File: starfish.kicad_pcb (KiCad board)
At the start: 2 copper layers, 40.5 x 25 mm, 35 parts, among them J1 microUSB, P1 CONN_02X05, P2 CONN_6X2, P3 CONN_2, U1 AP2120N, U2 SAMD21E15A-MU, U3 TPS73101, U4 FXMAR2104, U5 FXMAR2104, X1 CRYSTAL

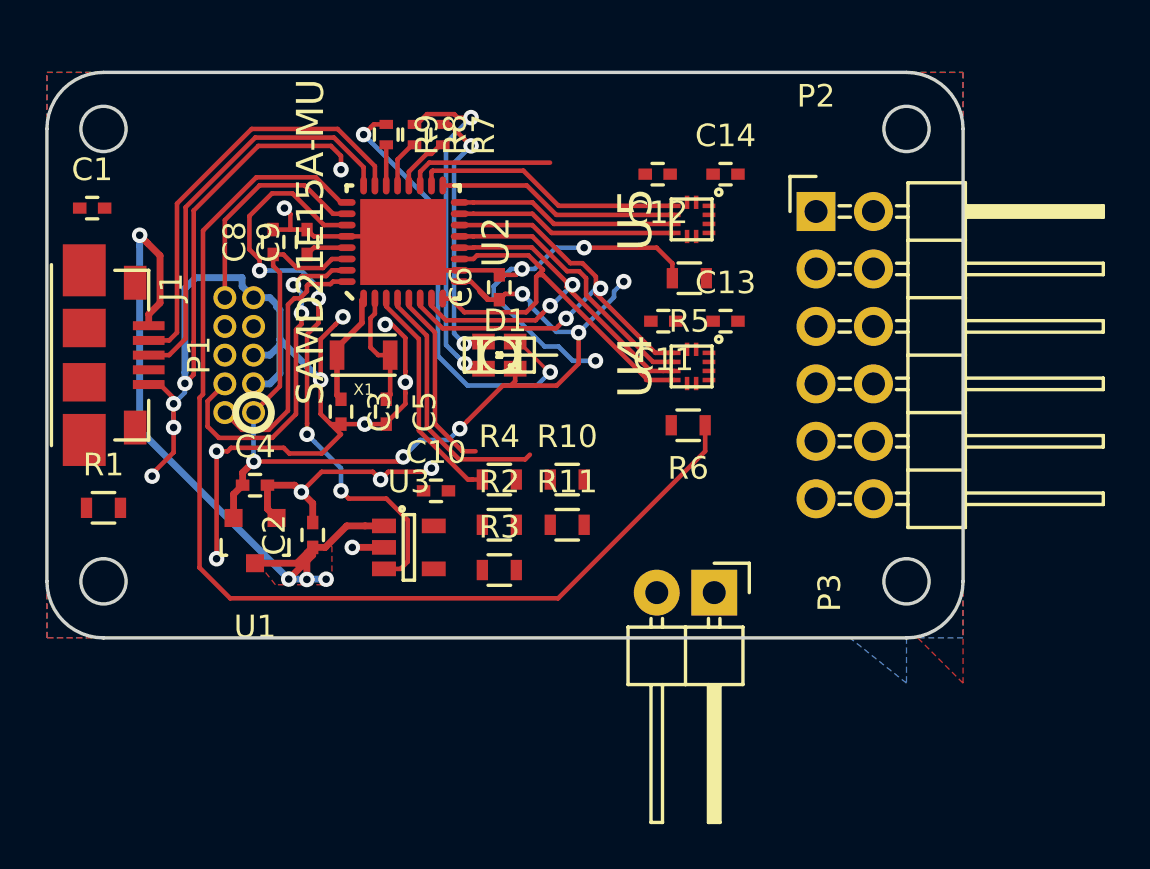
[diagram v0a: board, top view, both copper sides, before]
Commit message: Fully routed
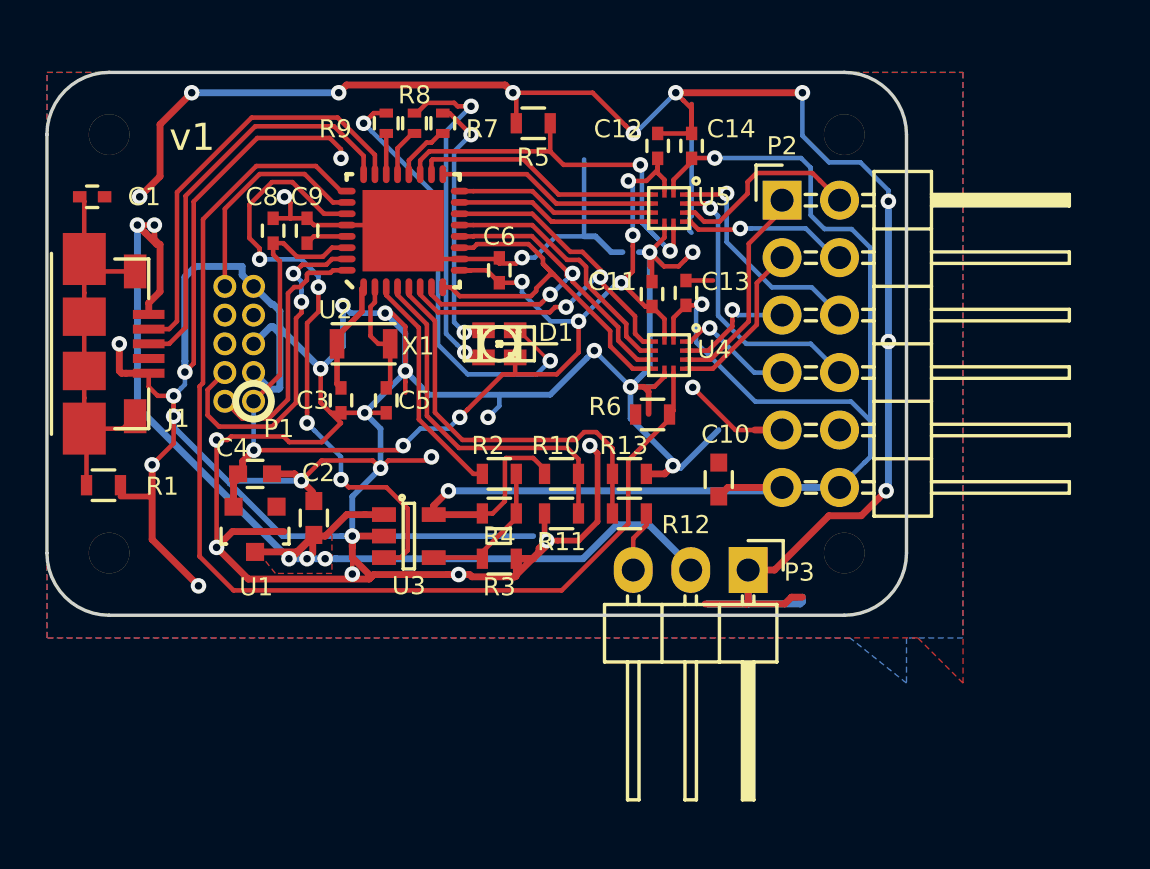
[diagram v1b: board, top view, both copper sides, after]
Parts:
- added R12: 47k, Resistors_SMD:R_0603, F.Cu at (125.8, 119.5)
- added R13: 27k, Resistors_SMD:R_0603, F.Cu at (125.8, 117.8)
- added REF**: MountingHole_M2, lib:MountingHole_M1.6, F.Cu at (135.2, 102.8)
- added REF**: MountingHole_M2, lib:MountingHole_M1.6, F.Cu at (102.8, 102.8)
- added REF**: MountingHole_M2, lib:MountingHole_M1.6, F.Cu at (102.8, 121.2)
- added REF**: MountingHole_M2, lib:MountingHole_M1.6, F.Cu at (135.2, 121.2)
- C10, C2, C4: footprint Capacitors_SMD:C_0402 -> Capacitors_SMD:C_0603
- P3: value CONN_2 -> CONN_3; footprint Pin_Headers:Pin_Header_Angled_1x02 -> Pin_Headers:Pin_Header_Angled_1x03
- R1, R10, R2: value R -> 47k
- R11, R3, R4, R5, R6: value R -> 27k
- moved C10 12.5 mm to (129.7, 118.0), turned to 90 degrees
- moved R5 9.72 mm to (121.5, 102.2)
- moved C13 2.15 mm to (128.2, 109.8), turned to 90 degrees
- moved C14 1.95 mm to (128.5, 103.2), turned to 90 degrees
- moved P3 1.80 mm to (131.0, 122.0)
- moved R6 1.65 mm to (126.8, 115.1)
- moved P2 1.58 mm to (132.5, 105.7)
- moved C11 1.30 mm to (126.8, 109.8), turned to 90 degrees
- moved C12 1.25 mm to (127.0, 103.2), turned to 90 degrees
- moved U4 1.12 mm to (127.5, 112.5)
- moved U5 1.12 mm to (127.5, 106.0)
- moved R1 1.00 mm to (102.5, 118.2)
- moved C2 0.75 mm to (111.8, 119.7)
- moved C6 0.75 mm to (120.0, 108.8)
- moved R11 0.56 mm to (122.8, 119.5), turned to 180 degrees
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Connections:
- net +3.3V renamed +3V3
- P1 pad 2: /SWCLK -> /SWDIO
- P1 pad 4: /SWDIO -> /SWCLK
- P3 pad 1: /ADC -> GND
- P3 pad 2: GND -> +5V
- U2 pad 15: /Y3M -> /Y2M
- U2 pad 16: /Y4M -> /Y1M
- U2 pad 17: /Y1M -> /Y4M
- U2 pad 18: /Y2M -> /Y3M
- U2 pad 31: /SWDIO -> /SWCLK
- U2 pad 32: /SWCLK -> /SWDIO
- U5 pad 10: /Y4 -> /Y1
- U5 pad 11: /Y1 -> /Y4
- U5 pad 12: /Y2 -> /Y3
- U5 pad 3: /Y2M -> /Y3M
- U5 pad 4: /Y1M -> /Y4M
- U5 pad 5: /Y4M -> /Y1M
- U5 pad 6: /Y3M -> /Y2M
- U5 pad 9: /Y3 -> /Y2
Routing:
- net GND: track 106.8 -> 313.3 mm, vias 20 -> 41
- net VAA: track 0.00 -> 66.8 mm, vias 0 -> 3
- net Net-(C1-Pad1): track 0.00 -> 18.3 mm
- net +5V: track 34.2 -> 52.3 mm, vias 4 -> 5
- net /EN_Y: track 6.51 -> 19.0 mm, vias 0 -> 2
- net /Y4: track 0.00 -> 12.5 mm, vias 0 -> 1
- net +3V3: track 45.0 -> 56.0 mm, vias 6 -> 8
- net /Y3: track 0.00 -> 10.3 mm, vias 0 -> 1
- net /ADC: track 8.31 -> 17.8 mm
- net /X1: track 0.00 -> 9.43 mm
- net /Y1: track 0.00 -> 8.97 mm
- net /Y2: track 0.00 -> 7.47 mm, vias 0 -> 1
- net /X2: track 0.00 -> 7.35 mm
- net Net-(R2-Pad2): track 0.00 -> 6.54 mm
- net /X3: track 0.00 -> 5.50 mm, vias 0 -> 1
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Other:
- board size 40.5 x 25 mm -> 38 x 24 mm
- rule pad_to_mask_clearance: 0.2 -> 0.0508
- board text added: "1 TXO CS"
- board text added: "1.2 - 5V"
- board text added: "2 RX MOSI"
- board text added: "3 SCL MISO"
- board text added: "4 SDA SCK"
- board text added: "B A"
- board text added: "GND"
- board text added: "GND 5V ADC"
- board text added: "v1"
